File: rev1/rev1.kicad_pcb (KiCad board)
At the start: 2 copper layers, 48.5 x 26.2 mm, 18 parts, among them J1 USB_C_Receptacle_USB2.0_14P, J2 P_IN, J3 DS3231, M1 Left, M2 Right, Q1 MMBT5551L, Q2 MMBT5551L, U1 ESP32-S3-WROOM-1, U2 DS18B20

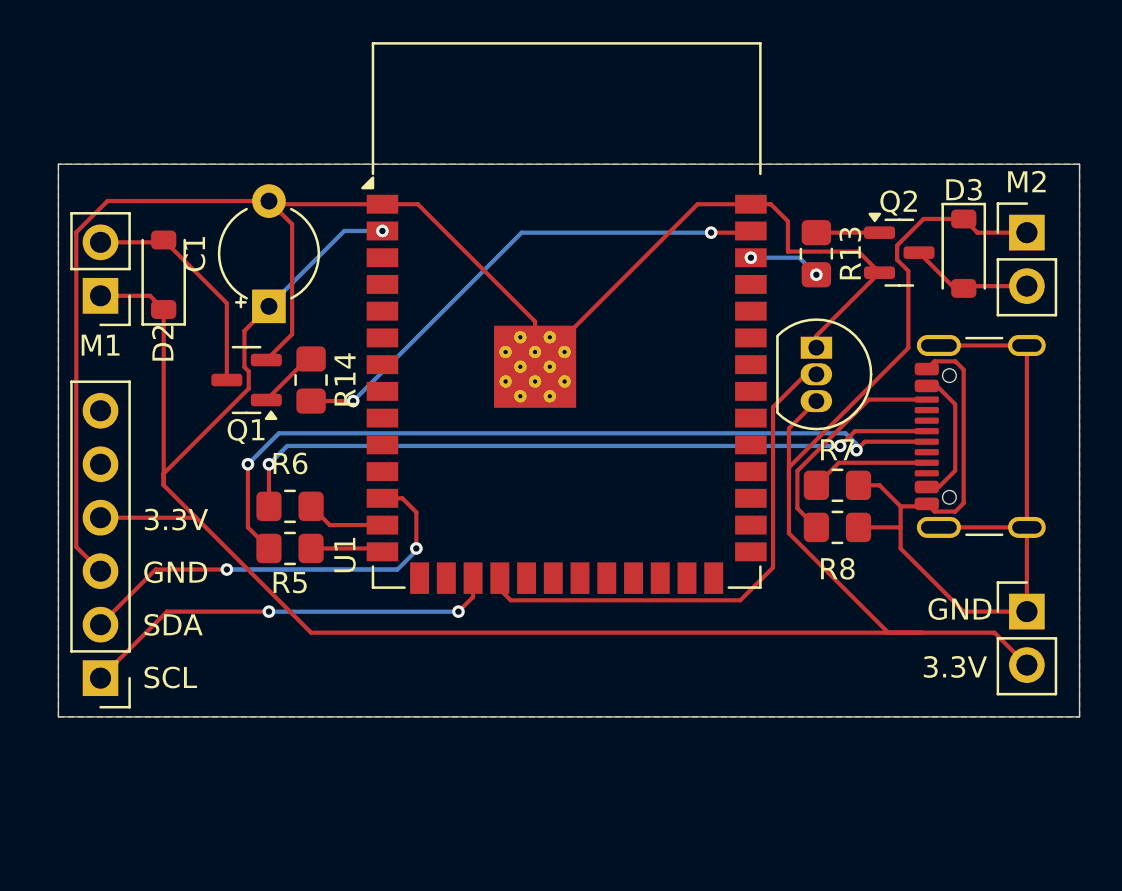
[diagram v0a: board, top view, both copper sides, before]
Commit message: Schematic and PCB project
Made with KiCad 9.0
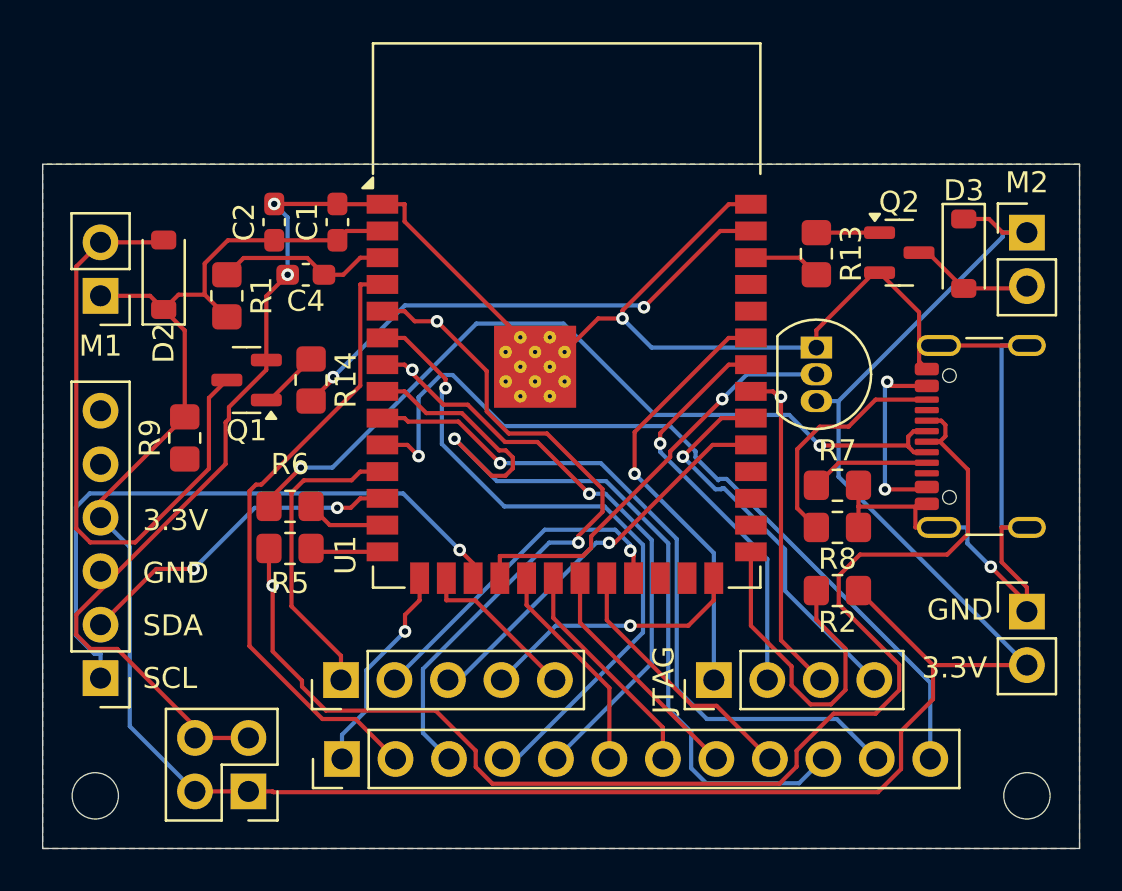
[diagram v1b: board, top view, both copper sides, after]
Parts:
- added C2: 22uF, Capacitor_SMD:C_0603_1608Metric_Pad1.08x0.95mm_HandSolder, F.Cu at (64.2, 78.5)
- added C4: 10uF, Capacitor_SMD:C_0603_1608Metric_Pad1.08x0.95mm_HandSolder, F.Cu at (65.8, 81.0)
- added J4: Conn_01x12_Pin, Connector_PinHeader_2.54mm:PinHeader_1x12_P2.54mm_Vertical, F.Cu at (67.5, 104.0)
- added J5: Conn_01x05_Pin, Connector_PinHeader_2.54mm:PinHeader_1x05_P2.54mm_Vertical, F.Cu at (67.4, 100.2)
- added J6: Conn_02x02_Counter_Clockwise, Connector_PinHeader_2.54mm:PinHeader_2x02_P2.54mm_Vertical, F.Cu at (63.0, 105.5)
- added JTAG: JTAG, Connector_PinHeader_2.54mm:PinHeader_1x04_P2.54mm_Vertical, F.Cu at (85.1, 100.2)
- added R1: 10k, Resistor_SMD:R_0805_2012Metric_Pad1.20x1.40mm_HandSolder, F.Cu at (62.0, 82.0)
- added R2: 10k, Resistor_SMD:R_0805_2012Metric_Pad1.20x1.40mm_HandSolder, F.Cu at (91.0, 96.0)
- added R9: 10k, Resistor_SMD:R_0805_2012Metric_Pad1.20x1.40mm_HandSolder, F.Cu at (60.0, 88.8)
- added REF**: MountingHole_2.2mm_M2, MountingHole:MountingHole_2.2mm_M2, F.Cu at (55.8, 105.8)
- added REF**: MountingHole_2.2mm_M2, MountingHole:MountingHole_2.2mm_M2, F.Cu at (100.0, 105.8)
- C1: footprint Capacitor_THT:CP_Radial_Tantal_D4.5mm_P5.00mm -> Capacitor_SMD:C_0603_1608Metric_Pad1.08x0.95mm_HandSolder
- R5, R6: value 22-33 -> 0
- moved C1 5.15 mm to (67.2, 78.5)
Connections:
- net 1 renamed M1
- net 2 renamed M2
- J1 pad B6: unconnected-(J1-D+-PadB6) -> Net-(J1-D+-PadA6)
- J1 pad B7: unconnected-(J1-D--PadB7) -> Net-(J1-D--PadA7)
- U1 pad 24: 47 -> unconnected-(U1-IO47-Pad24)
- U1 pad 25: 48 -> unconnected-(U1-IO48-Pad25)
- U1 pad 27: unconnected-(U1-IO0-Pad27) -> Net-(U1-IO0)
- U1 pad 3: unconnected-(U1-EN-Pad3) -> EN
- U1 pad 32: 39 -> Net-(J7-Pin_4)
- U1 pad 33: 40 -> Net-(J7-Pin_3)
- U1 pad 34: 41 -> Net-(J7-Pin_2)
- U1 pad 35: 42 -> Net-(J7-Pin_1)
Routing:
- net 15: track 0.00 -> 42.0 mm, vias 0 -> 1
- net 17: track 0.00 -> 39.4 mm, vias 0 -> 1
- net 16: track 0.00 -> 34.4 mm, vias 0 -> 1
- net 5: track 0.00 -> 32.8 mm, vias 0 -> 2
- net 6: track 0.00 -> 31.8 mm, vias 0 -> 1
- net 4: track 0.00 -> 29.7 mm
- net 7: track 0.00 -> 28.6 mm, vias 0 -> 2
- net Net-(J1-D+-PadA6): track 37.9 -> 61.2 mm, vias 2 -> 1
- net Net-(J7-Pin_1): track 0.00 -> 20.7 mm, vias 0 -> 1
- net Net-(J7-Pin_2): track 0.00 -> 19.5 mm, vias 0 -> 1
- net 38: track 0.00 -> 19.0 mm, vias 0 -> 1
- net Net-(D2-A): track 10.9 -> 29.7 mm
- net Net-(J7-Pin_4): track 0.00 -> 18.7 mm, vias 0 -> 1
- net 21: track 0.00 -> 16.1 mm, vias 0 -> 1
- net Net-(J7-Pin_3): track 0.00 -> 15.8 mm, vias 0 -> 1
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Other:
- board size 48.5 x 26.2 mm -> 49.2 x 32.5 mm
